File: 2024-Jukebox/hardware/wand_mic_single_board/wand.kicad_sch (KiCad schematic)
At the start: 50 parts, among them J1 USB_C_Receptacle_USB2.0, J10 Conn_01x03, J4 Conn_01x02, J6 Conn_01x01, J9 Conn_01x02, Q1 MUN5214DW1T1G, Q3 CJ3139K, U1 CP2104, U2 ESP32-PICO-D4, U3 ICM-20948, U4 TP4065-4.2V, U5 TLV76718DRVx, U6 LY68L6400SLIT, U7 PCA9306, U9 TLV76733DRVx

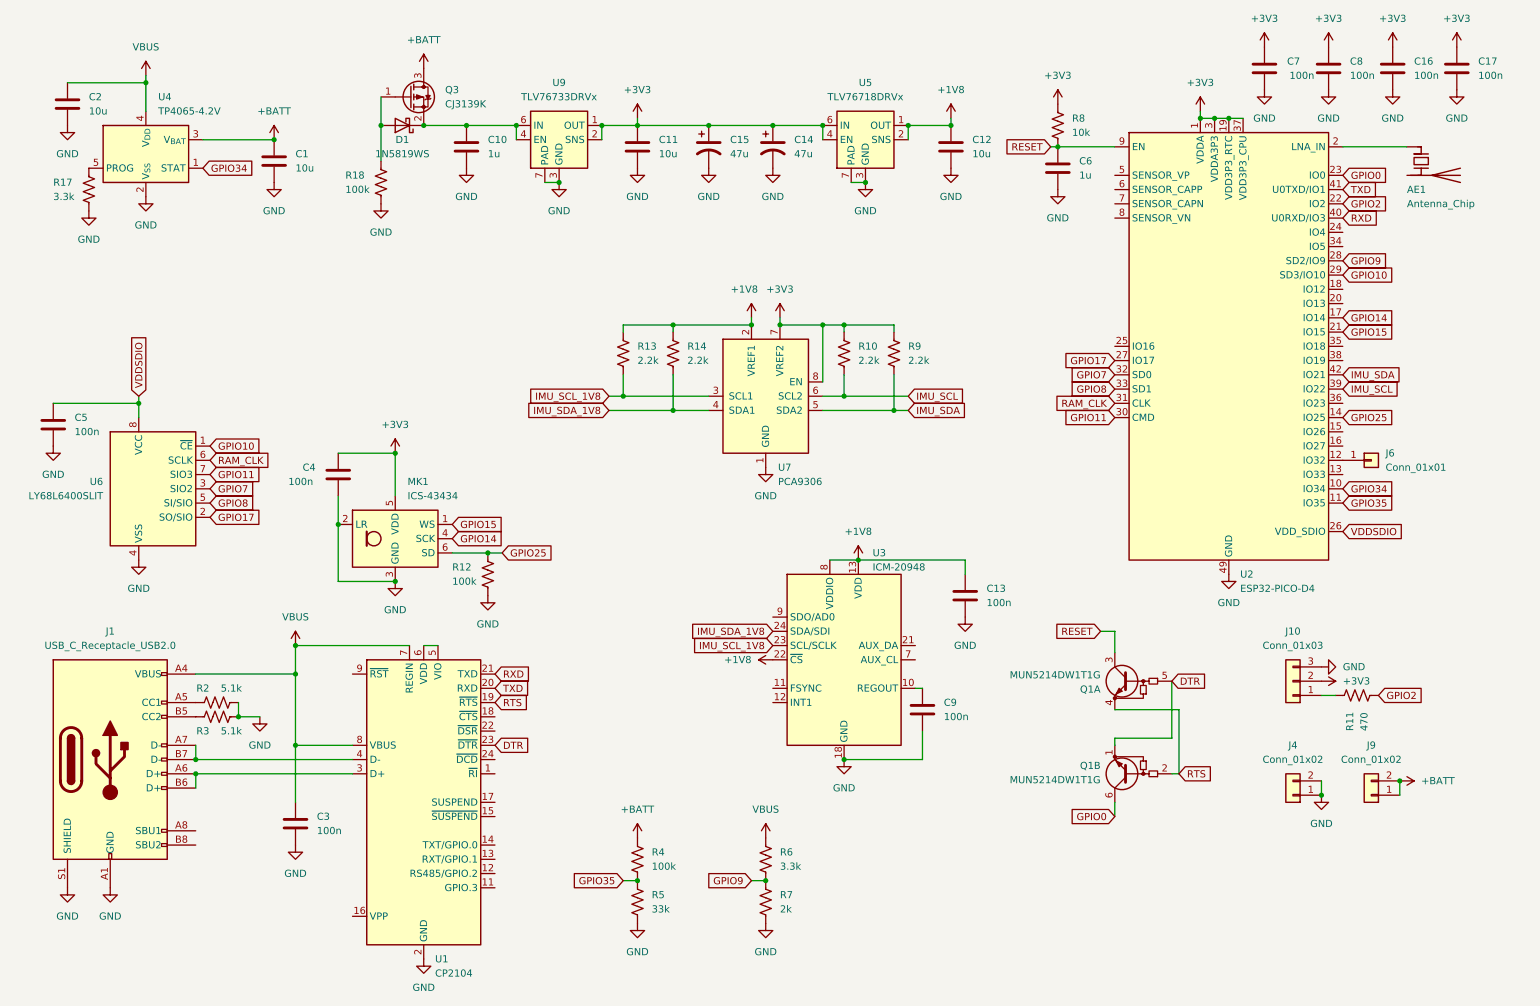
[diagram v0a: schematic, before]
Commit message: Updated wand PCBs
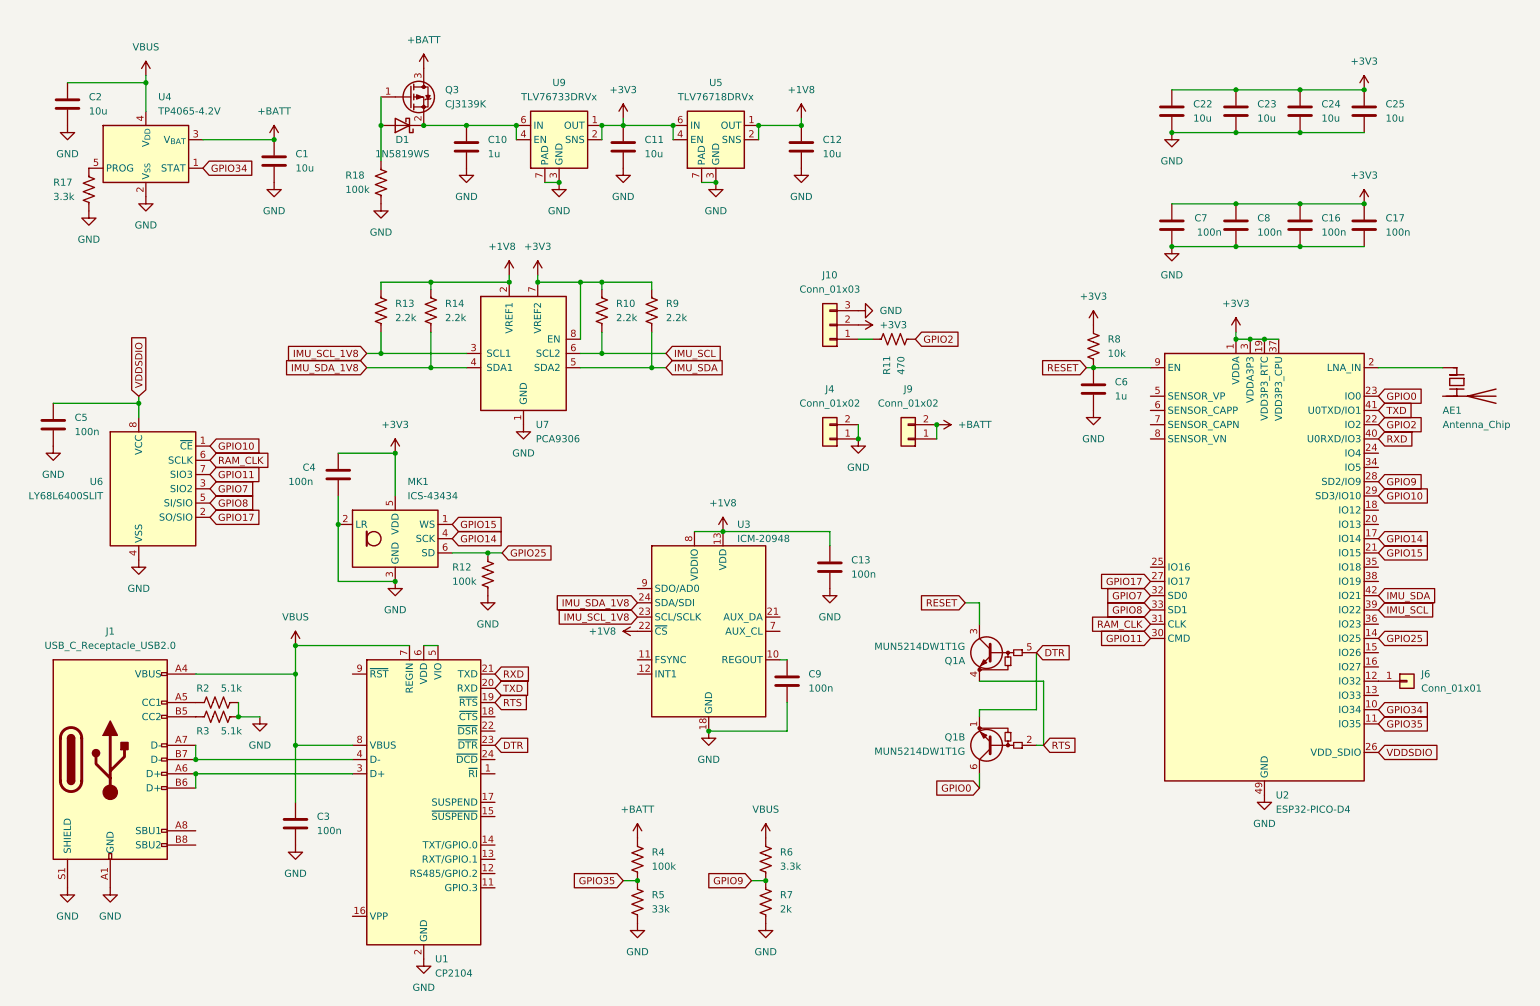
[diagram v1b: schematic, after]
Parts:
- removed C14, C15: 47u, Capacitor_SMD:C_0805_2012Metric, symbol Device:C_Polarized_US
- added C22, C23, C24, C25: 10u, Capacitor_SMD:C_0402_1005Metric, symbol Device:C
- C9: footprint Capacitor_SMD:C_0402_1005Metric -> Capacitor_SMD:C_0603_1608Metric
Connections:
- net +3V3: now also C22.1, C23.1, C24.1, C25.1
- net GND: now also C22.2, C23.2, C24.2, C25.2
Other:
- moved on the sheet: AE1, C11, C12, C13, C16, C17, C6, C7, C8, C9, J10, J4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
